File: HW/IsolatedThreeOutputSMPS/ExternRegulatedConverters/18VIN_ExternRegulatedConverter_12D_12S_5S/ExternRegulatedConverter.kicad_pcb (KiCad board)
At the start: 2 copper layers, 71.1 x 47 mm, 20 parts, among them J1 15VDC, J2 Conn_01x07, U1 RS6-1212D, U2 LM7805_TO220, U3 LM7812_TO220, U4 LM7912_TO220, U5 LM7812_TO220

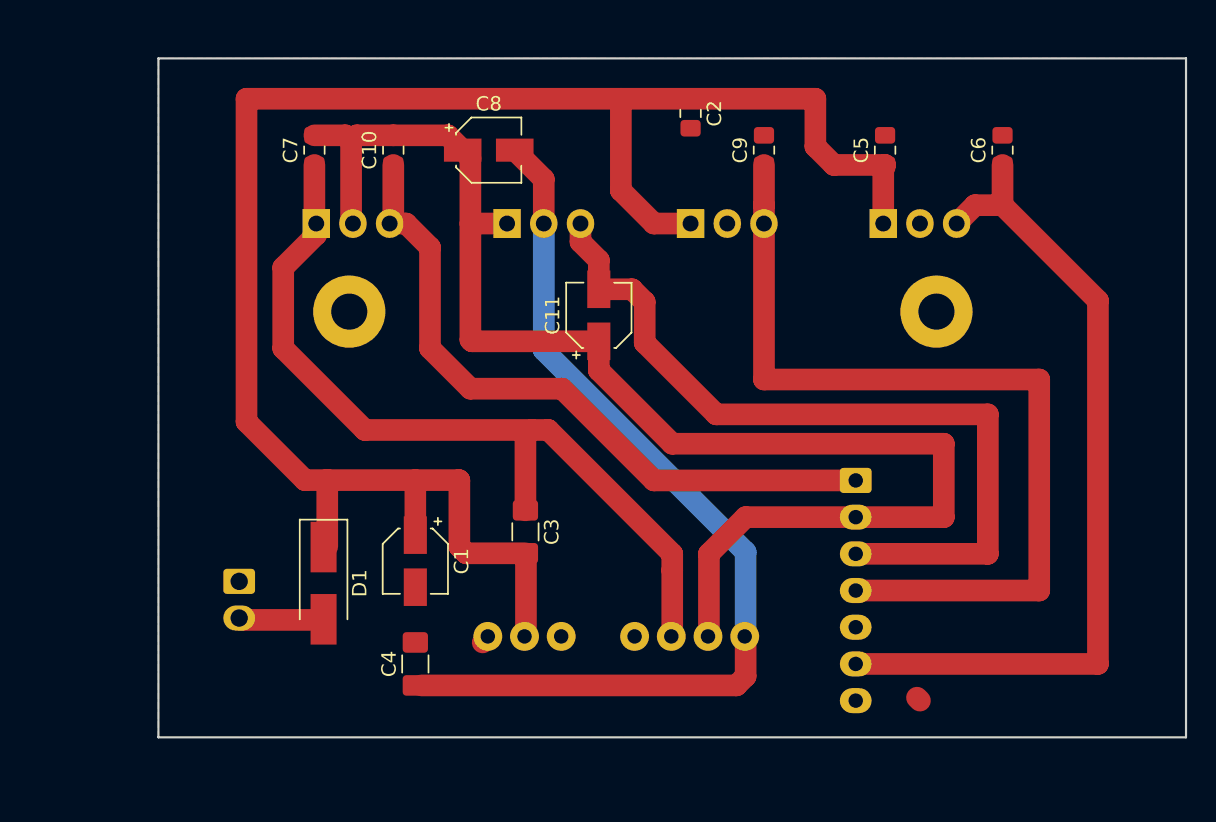
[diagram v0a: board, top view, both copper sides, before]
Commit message: RevA layout PSU
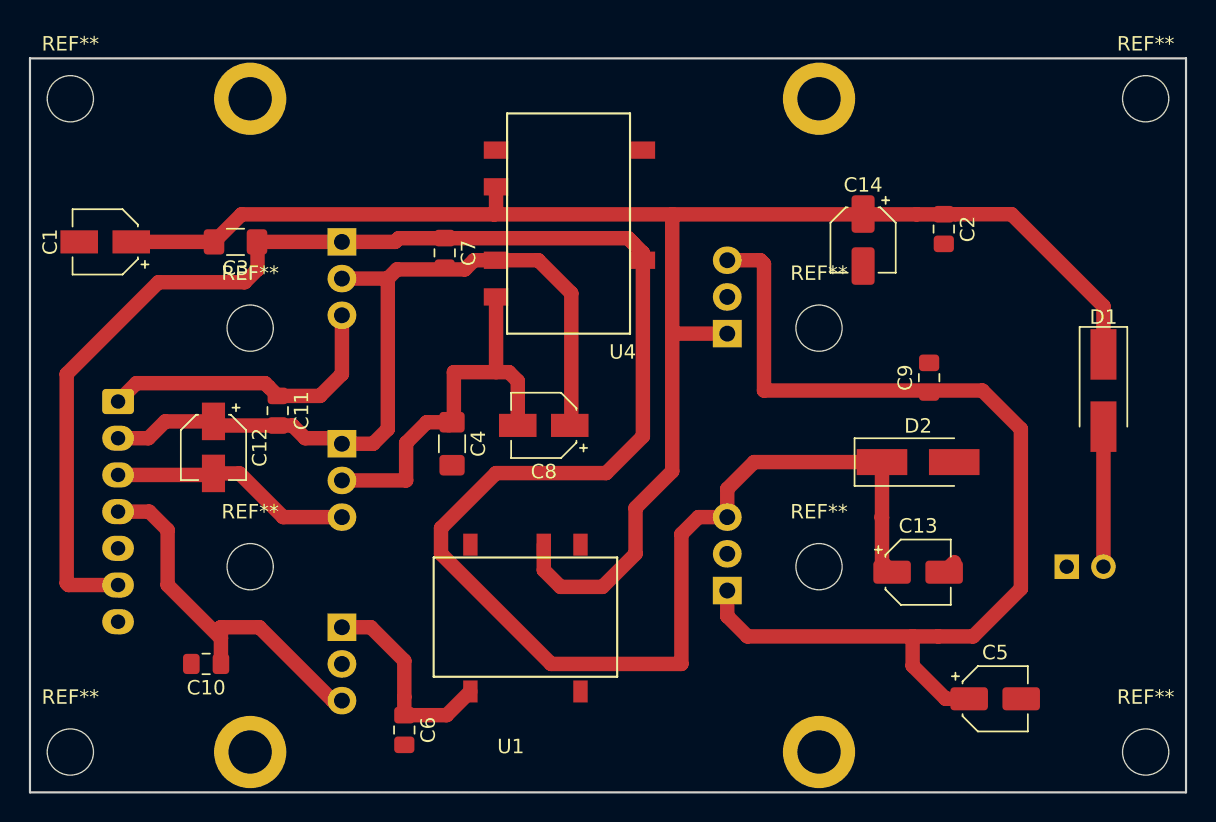
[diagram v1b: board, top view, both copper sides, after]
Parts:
- added C10: 100nF, Capacitor_SMD:C_0805_2012Metric_Pad1.15x1.40mm_HandSolder, F.Cu at (104.9, 114.3)
- added C13: 1uF, Capacitor_SMD:CP_Elec_4x5.7, F.Cu at (154.2, 108.0)
- added C14: 4.7uF, Capacitor_SMD:CP_Elec_4x5.7, F.Cu at (150.4, 85.0)
- added D2: ES2G, Diode_SMD:D_SMA_Handsoldering, F.Cu at (154.2, 100.3)
- added HS2: Heatsink, Heatsink:Heatsink_SheetType_50x7mm_2Fixations, B.Cu at (108.0, 97.8)
- added REF**: MountingHole_3.2mm_M3_DIN965, MountingHole:MountingHole_3.2mm_M3_DIN965, F.Cu at (108.0, 91.1)
- added REF**: MountingHole_3.2mm_M3_DIN965, MountingHole:MountingHole_3.2mm_M3_DIN965, F.Cu at (108.0, 107.6)
- added REF**: MountingHole_3.2mm_M3_DIN965, MountingHole:MountingHole_3.2mm_M3_DIN965, F.Cu at (147.3, 91.1)
- added REF**: MountingHole_3.2mm_M3_DIN965, MountingHole:MountingHole_3.2mm_M3_DIN965, F.Cu at (147.3, 107.6)
- added REF**: MountingHole_3.2mm_M3_DIN965, MountingHole:MountingHole_3.2mm_M3_DIN965, F.Cu at (169.9, 75.2)
- added REF**: MountingHole_3.2mm_M3_DIN965, MountingHole:MountingHole_3.2mm_M3_DIN965, F.Cu at (169.9, 120.4)
- added REF**: MountingHole_3.2mm_M3_DIN965, MountingHole:MountingHole_3.2mm_M3_DIN965, F.Cu at (95.5, 120.4)
- added REF**: MountingHole_3.2mm_M3_DIN965, MountingHole:MountingHole_3.2mm_M3_DIN965, F.Cu at (95.5, 75.2)
- added U6: L7818CV, Package_TO_SOT_THT:TO-220-3_Vertical, B.Cu at (141.0, 91.4)
- added U7: L78M15ABV, Package_TO_SOT_THT:TO-220-3_Vertical, B.Cu at (141.0, 109.2)
- C1: value 2.2uF -> 4.7uF
- C12: renamed from C11; value 10uF -> 1uF
- C5: value 330nF -> 100nF; footprint Capacitor_SMD:C_0805_2012Metric_Pad1.15x1.40mm_HandSolder -> Capacitor_SMD:CP_Elec_4x5.7
- C6, C9: value 100nF -> 330nF
- C8: value 10uF -> 2.2uF
- D1: value D_Schottky -> BYS12-90-E3/TR
- HS1: value Heatsink -> Heatsink 6.8K/W
- J1: footprint Connector_Molex:Molex_KK-254_AE-6410-02A_1x02_P2.54mm_Vertical -> Connector_PinHeader_2.54mm:PinHeader_1x02_P2.54mm_Horizontal
- U1: value RS6-1212D -> ISE2409A-H; footprint ITX1212S:ITX1212S -> XPower_Converter_DCDC:ISE; moved to F.Cu
- U2: value LM7805_TO220 -> LM7812_TO220
- U3: value LM7812_TO220 -> LM7912_TO220
- U4: value LM7912_TO220 -> R2D-2415; footprint Package_TO_SOT_THT:TO-220-3_Vertical -> RS6:R2D; moved to F.Cu
- U5: value LM7812_TO220 -> LM7805_TO220
- moved C6 57.7 mm to (118.6, 118.9), turned to 270 degrees
- moved J1 57.3 mm to (164.5, 107.6)
- moved D1 55.6 mm to (167.0, 95.4)
- moved J2 51.3 mm to (98.8, 96.1)
- moved U5 46.7 mm to (114.3, 111.8), turned to 270 degrees
- moved C5 38.7 mm to (159.5, 116.7), turned to 0 degrees
- moved C1 30.8 mm to (97.9, 85.1), turned to 180 degrees
- moved C3 28.4 mm to (106.9, 85.1), turned to 180 degrees
- moved C12 28.2 mm to (105.4, 99.3), turned to 270 degrees
- moved U2 24.2 mm to (114.3, 85.1), turned to 270 degrees
- moved C11 19.7 mm to (109.9, 96.8), turned to 270 degrees
- moved C9 19.5 mm to (154.9, 94.5)
- moved C8 19.4 mm to (128.3, 97.8), turned to 180 degrees
- moved C2 19.3 mm to (156.0, 84.2)
- moved C4 15.5 mm to (121.9, 99.1), turned to 270 degrees
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- renumbered C10 to C11
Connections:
- C1 pad 1: +15V -> +24V
- C1 pad 2: GNDA -> GNDS
- C2 pad 1: +15V -> +24V
- C2 pad 2: GNDA -> GNDS
- C3 pad 1: Net-(C3-Pad1) -> +15V
- C3 pad 2: +15V -> +24V
- C4 pad 1: Net-(C4-Pad1) -> /-15V
- C4 pad 2: GNDA -> GNDS
- C5 pad 1: +15V -> /+18V
- C5 pad 2: GNDA -> GNDS
- C6 pad 1: +12P -> /+9V
- C6 pad 2: GNDA -> GNDS
- C7 pad 1: Net-(C3-Pad1) -> +15V
- C8 pad 2: Net-(C4-Pad1) -> /-15V
- C9 pad 1: +5V -> /+18V
- C9 pad 2: GNDA -> GNDS
- D1 pad 1: +15V -> +24V
- J1 pad 1: GNDA -> GNDS
- J2 pad 5: GNDA -> GNDS
- J2 pad 6: +12P -> +15V
- J2 pad 7: GNDA -> GNDS
- U1 pad 1: GNDA -> GNDS
- U1 pad 2: +15V -> +24V
- U1 pad 5: (no net) -> /+9V
- U1 pad 8: Net-(C4-Pad1) -> (no net)
- U2 pad 2: GNDA -> VCOM
- U2 pad 3: +5V -> +12V
- U3 pad 1: Net-(C3-Pad1) -> VCOM
- U3 pad 2: VCOM -> /-15V
- U3 pad 3: +12V -> -12V
- U4 pad 1: VCOM -> GNDS
- U4 pad 2: Net-(C4-Pad1) -> +24V
- U5 pad 1: +15V -> /+9V
- U5 pad 2: GNDA -> GNDS
- U5 pad 3: +12P -> +5V
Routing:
- net +24V: track 0.00 -> 114.1 mm
- net /+18V: track 0.00 -> 72.3 mm
- net Net-(C4-Pad1): track 65.7 -> 0.00 mm
- net Net-(C3-Pad1): track 58.0 -> 0.00 mm
- net +12P: track 57.7 -> 0.00 mm
- net VCOM: track 97.7 -> 57.2 mm
- net -12V: track 56.0 -> 16.8 mm
- net +5V: track 61.2 -> 26.2 mm
- net /-15V: track 0.00 -> 27.6 mm
- net +12V: track 48.1 -> 21.1 mm
- net +15V: track 126.5 -> 149.0 mm
- net /+9V: track 0.00 -> 14.3 mm
- net Net-(D1-Pad2): track 5.91 -> 9.56 mm
- net GNDS: track 0.00 -> 1.35 mm
- net GNDA: track 0.88 -> 0.00 mm
- added copper zone on F.Cu, net GNDS
- removed copper zone on F.Cu, net GNDA
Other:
- board size 71.1 x 47 mm -> 80 x 50.8 mm
